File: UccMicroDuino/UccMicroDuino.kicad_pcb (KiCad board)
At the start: 2 copper layers, 14 parts, among them J1 USB_PCB_A, J2 Header, U1 ATtiny85-20S

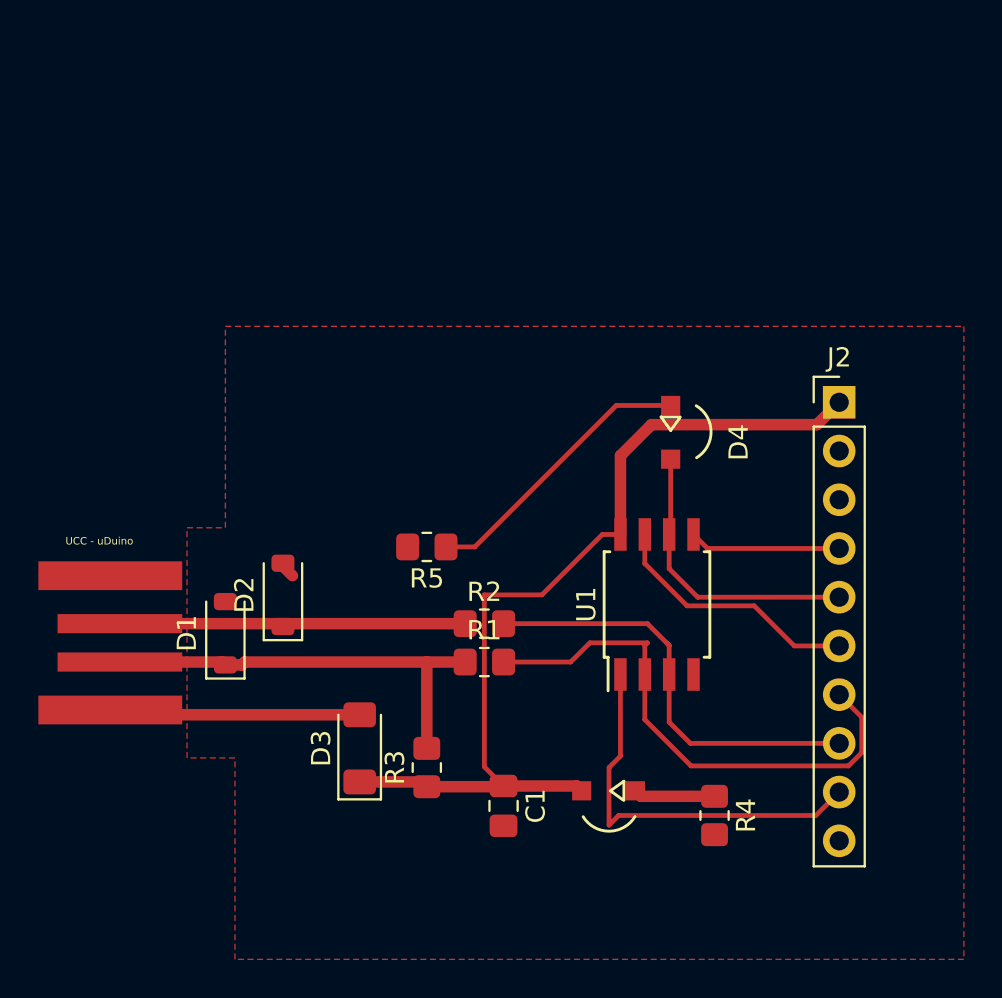
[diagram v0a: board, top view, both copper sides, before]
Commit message: 18-05-2026
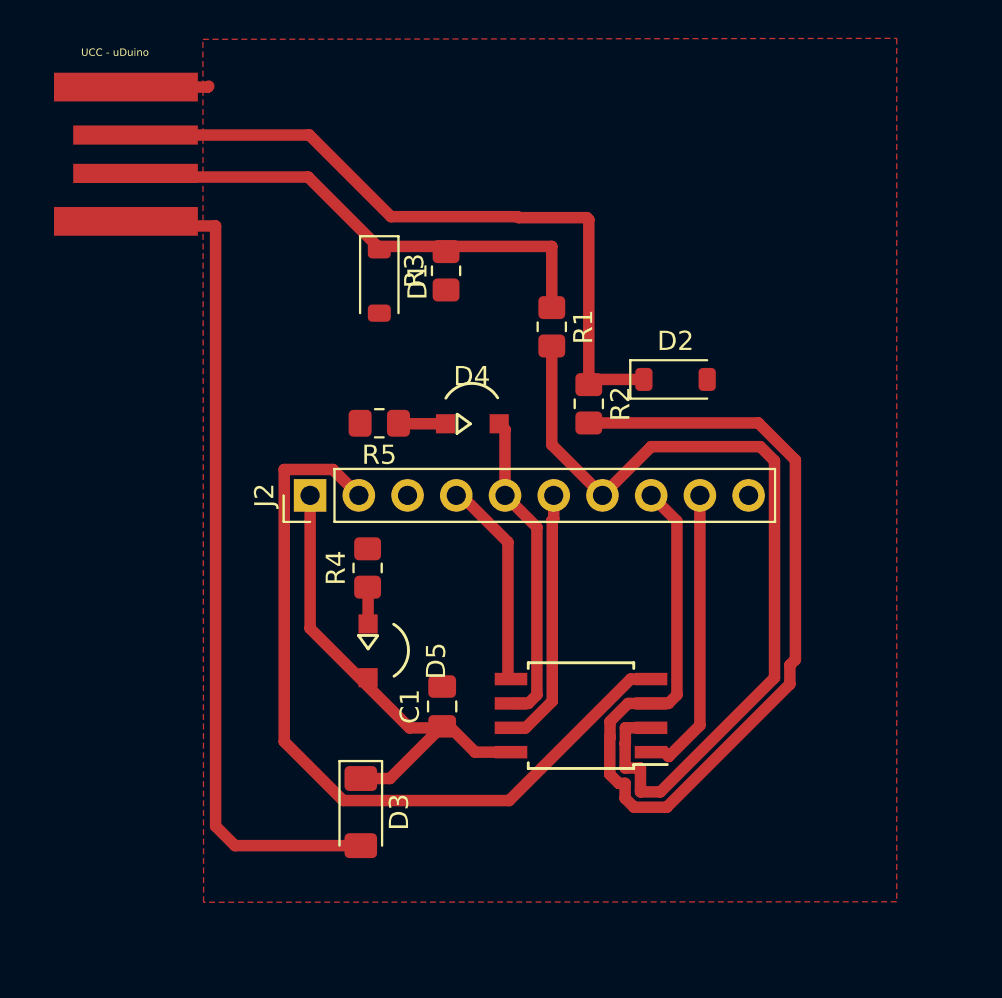
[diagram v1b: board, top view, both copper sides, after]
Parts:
- moved J2 28.0 mm to (134.4, 73.8), turned to 90 degrees
- moved R3 25.9 mm to (141.5, 62.1)
- moved J1 25.5 mm to (125.0, 56.0)
- moved D2 23.3 mm to (153.5, 67.8), turned to 0 degrees
- moved R4 22.2 mm to (137.4, 77.6), turned to 90 degrees
- moved D1 20.0 mm to (138.0, 62.7), turned to -90 degrees
- moved R1 17.8 mm to (147.0, 65.0), turned to -90 degrees
- moved D5 14.0 mm to (137.4, 82.3), turned to -90 degrees
- moved R2 12.7 mm to (148.9, 69.0), turned to -90 degrees
- moved D4 9.97 mm to (143.3, 70.1), turned to 0 degrees
- moved U1 7.02 mm to (148.5, 85.3), turned to 180 degrees
- moved R5 6.91 mm to (138.0, 70.1)
- moved C1 6.09 mm to (141.3, 84.8), turned to 90 degrees
- moved D3 3.32 mm to (137.1, 90.3), turned to -90 degrees
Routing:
- net GND: track 1.72 -> 46.4 mm
- net Net-(J2-Pin_8): track 22.8 -> 54.4 mm
- net Net-(D3-A): track 13.1 -> 44.1 mm
- net +5V: track 47.2 -> 25.4 mm
- net Net-(D2-K): track 18.0 -> 37.0 mm
- net Net-(J2-Pin_7): track 28.1 -> 45.6 mm
- net Net-(D4-K): track 14.8 -> 2.46 mm
- net Net-(J2-Pin_9): track 20.8 -> 15.3 mm
- net Net-(D1-K): track 22.6 -> 26.5 mm
- net Net-(J2-Pin_4): track 7.90 -> 10.9 mm
- net Net-(D5-K): track 4.24 -> 1.93 mm
- net Net-(D4-A): track 15.2 -> 16.5 mm
